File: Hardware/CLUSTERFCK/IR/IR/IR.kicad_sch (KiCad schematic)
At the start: 40 parts, among them J1 Conn_02x20_Counter_Clockwise, J2 Conn_02x20_Counter_Clockwise, U1 74LS08, U2 74HCT574, U3 74HCT574

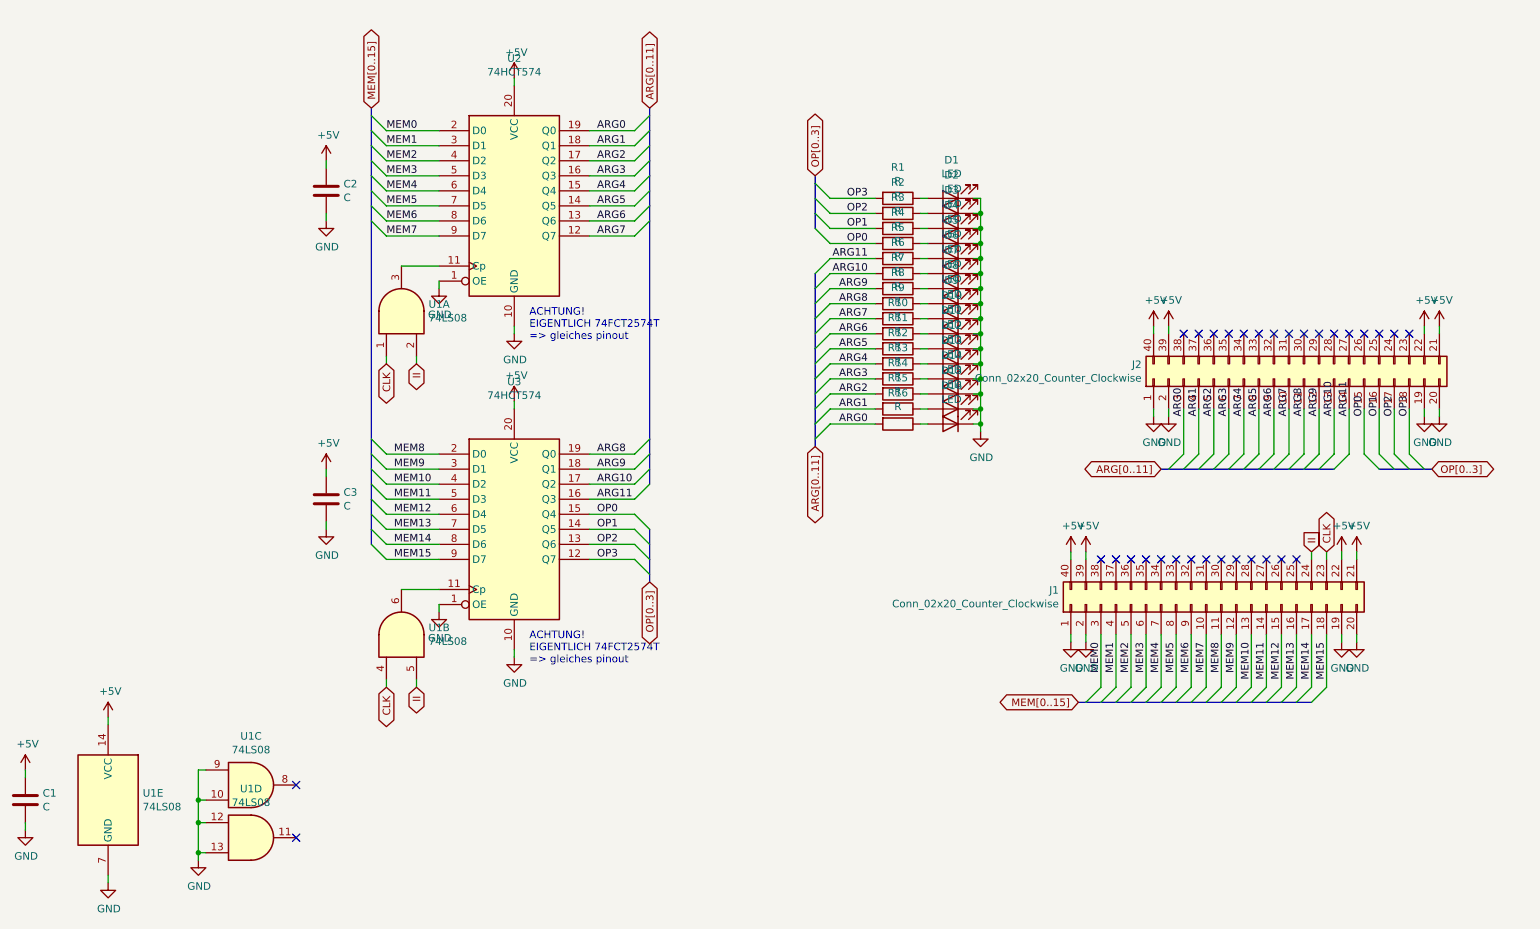
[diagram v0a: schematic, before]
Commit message: 0065 | 24h | ADDR & DATA & PLACEHOLDER etc
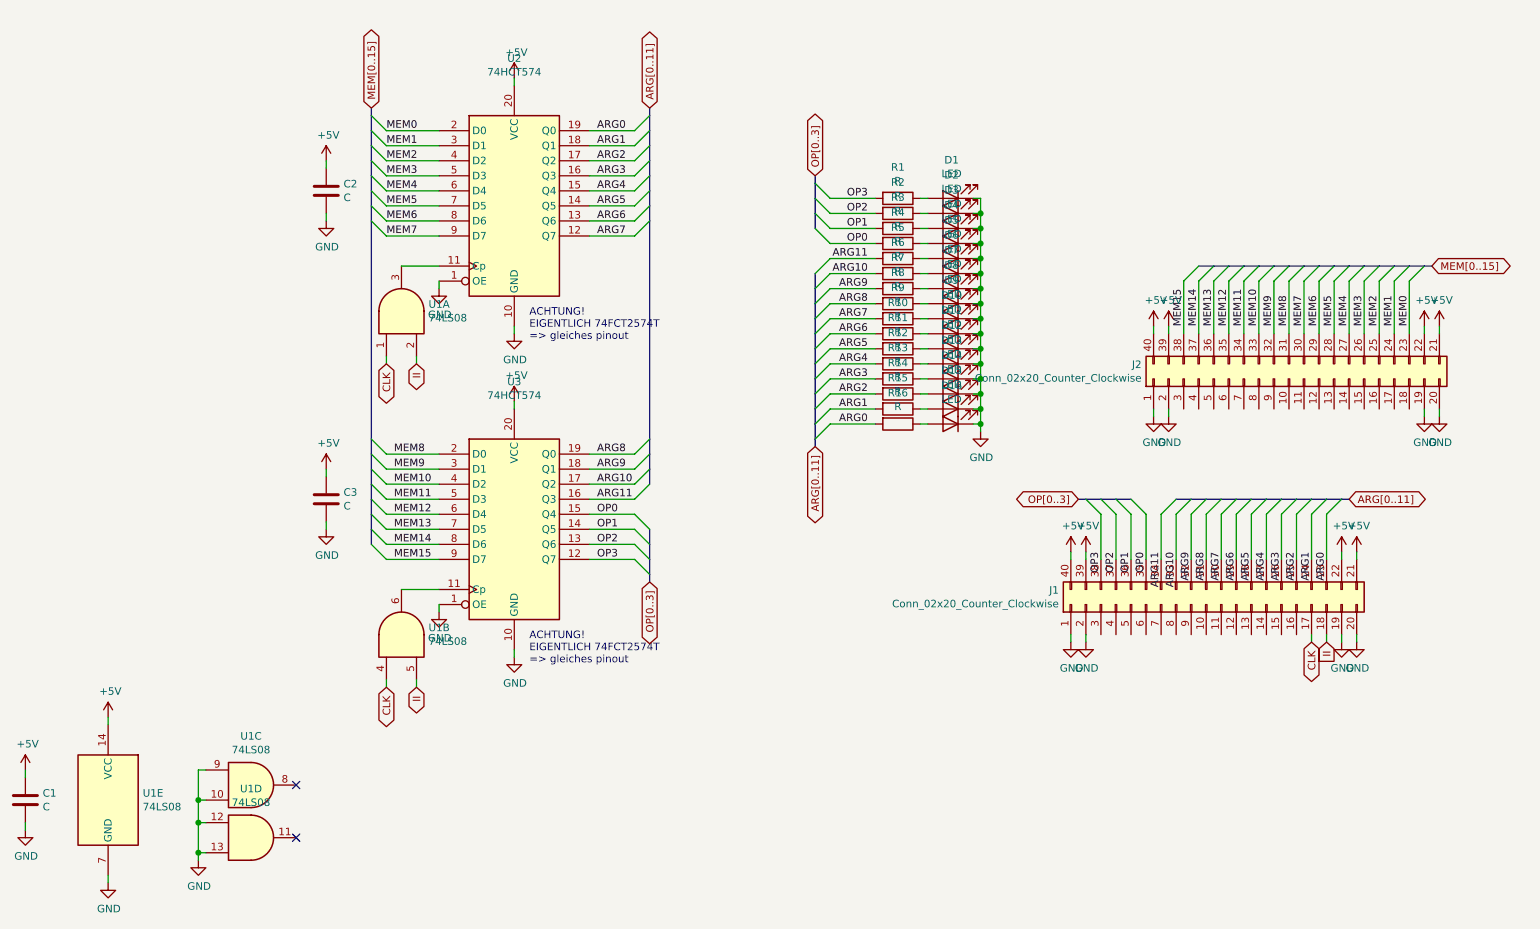
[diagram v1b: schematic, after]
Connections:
- net ARG0: now also J1.23 (Pin_23); no longer J2.3 (Pin_3)
- net ARG1: now also J1.24 (Pin_24); no longer J2.4 (Pin_4)
- net ARG10: now also J1.33 (Pin_33); no longer J2.13 (Pin_13)
- net ARG11: now also J1.34 (Pin_34); no longer J2.14 (Pin_14)
- net ARG2: now also J1.25 (Pin_25); no longer J2.5 (Pin_5)
- net ARG3: now also J1.26 (Pin_26); no longer J2.6 (Pin_6)
- net ARG4: now also J1.27 (Pin_27); no longer J2.7 (Pin_7)
- net ARG5: now also J1.28 (Pin_28); no longer J2.8 (Pin_8)
- net ARG6: now also J1.29 (Pin_29); no longer J2.9 (Pin_9)
- net ARG7: now also J1.30 (Pin_30); no longer J2.10 (Pin_10)
- net ARG8: now also J1.31 (Pin_31); no longer J2.11 (Pin_11)
- net ARG9: now also J1.32 (Pin_32); no longer J2.12 (Pin_12)
- net CLK: now also J1.17 (Pin_17); no longer J1.23 (Pin_23)
- net II: now also J1.18 (Pin_18); no longer J1.24 (Pin_24)
- net MEM0: now also J2.23 (Pin_23); no longer J1.3 (Pin_3)
- net MEM1: now also J2.24 (Pin_24); no longer J1.4 (Pin_4)
- net MEM10: now also J2.33 (Pin_33); no longer J1.13 (Pin_13)
- net MEM11: now also J2.34 (Pin_34); no longer J1.14 (Pin_14)
- net MEM12: now also J2.35 (Pin_35); no longer J1.15 (Pin_15)
- net MEM13: now also J2.36 (Pin_36); no longer J1.16 (Pin_16)
- net MEM14: now also J2.37 (Pin_37); no longer J1.17 (Pin_17)
- net MEM15: now also J2.38 (Pin_38); no longer J1.18 (Pin_18)
- net MEM2: now also J2.25 (Pin_25); no longer J1.5 (Pin_5)
- net MEM3: now also J2.26 (Pin_26); no longer J1.6 (Pin_6)
- net MEM4: now also J2.27 (Pin_27); no longer J1.7 (Pin_7)
- net MEM5: now also J2.28 (Pin_28); no longer J1.8 (Pin_8)
- net MEM6: now also J2.29 (Pin_29); no longer J1.9 (Pin_9)
- net MEM7: now also J2.30 (Pin_30); no longer J1.10 (Pin_10)
- net MEM8: now also J2.31 (Pin_31); no longer J1.11 (Pin_11)
- net MEM9: now also J2.32 (Pin_32); no longer J1.12 (Pin_12)
- net OP0: now also J1.35 (Pin_35); no longer J2.15 (Pin_15)
- net OP1: now also J1.36 (Pin_36); no longer J2.16 (Pin_16)
- net OP2: now also J1.37 (Pin_37); no longer J2.17 (Pin_17)
- net OP3: now also J1.38 (Pin_38); no longer J2.18 (Pin_18)
- no-connect marks 32 -> 2
